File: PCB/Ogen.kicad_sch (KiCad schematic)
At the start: 17 parts, among them J1 Input, U1 PMW3360DM-T2QU, U2 TLV70019, U3 TXS0102DCU, U4 TXS0102DCU, U5 TXS0102DCU

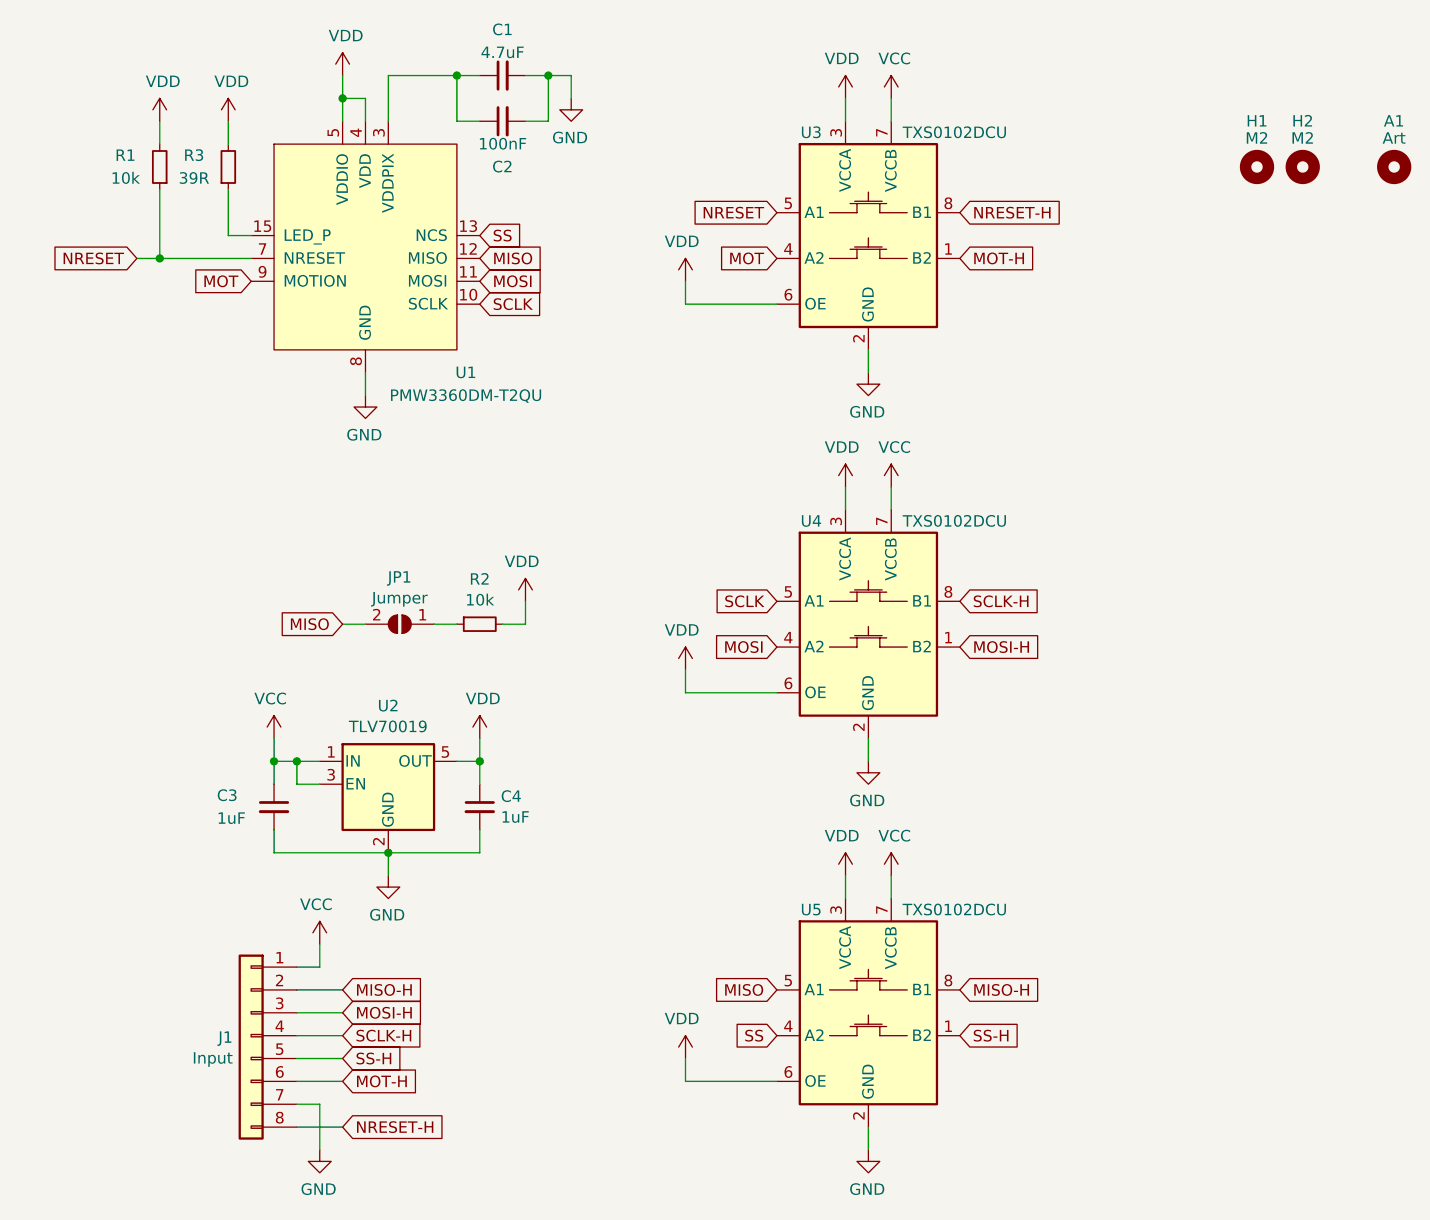
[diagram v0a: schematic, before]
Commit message: V1.0 Lite initial commit.
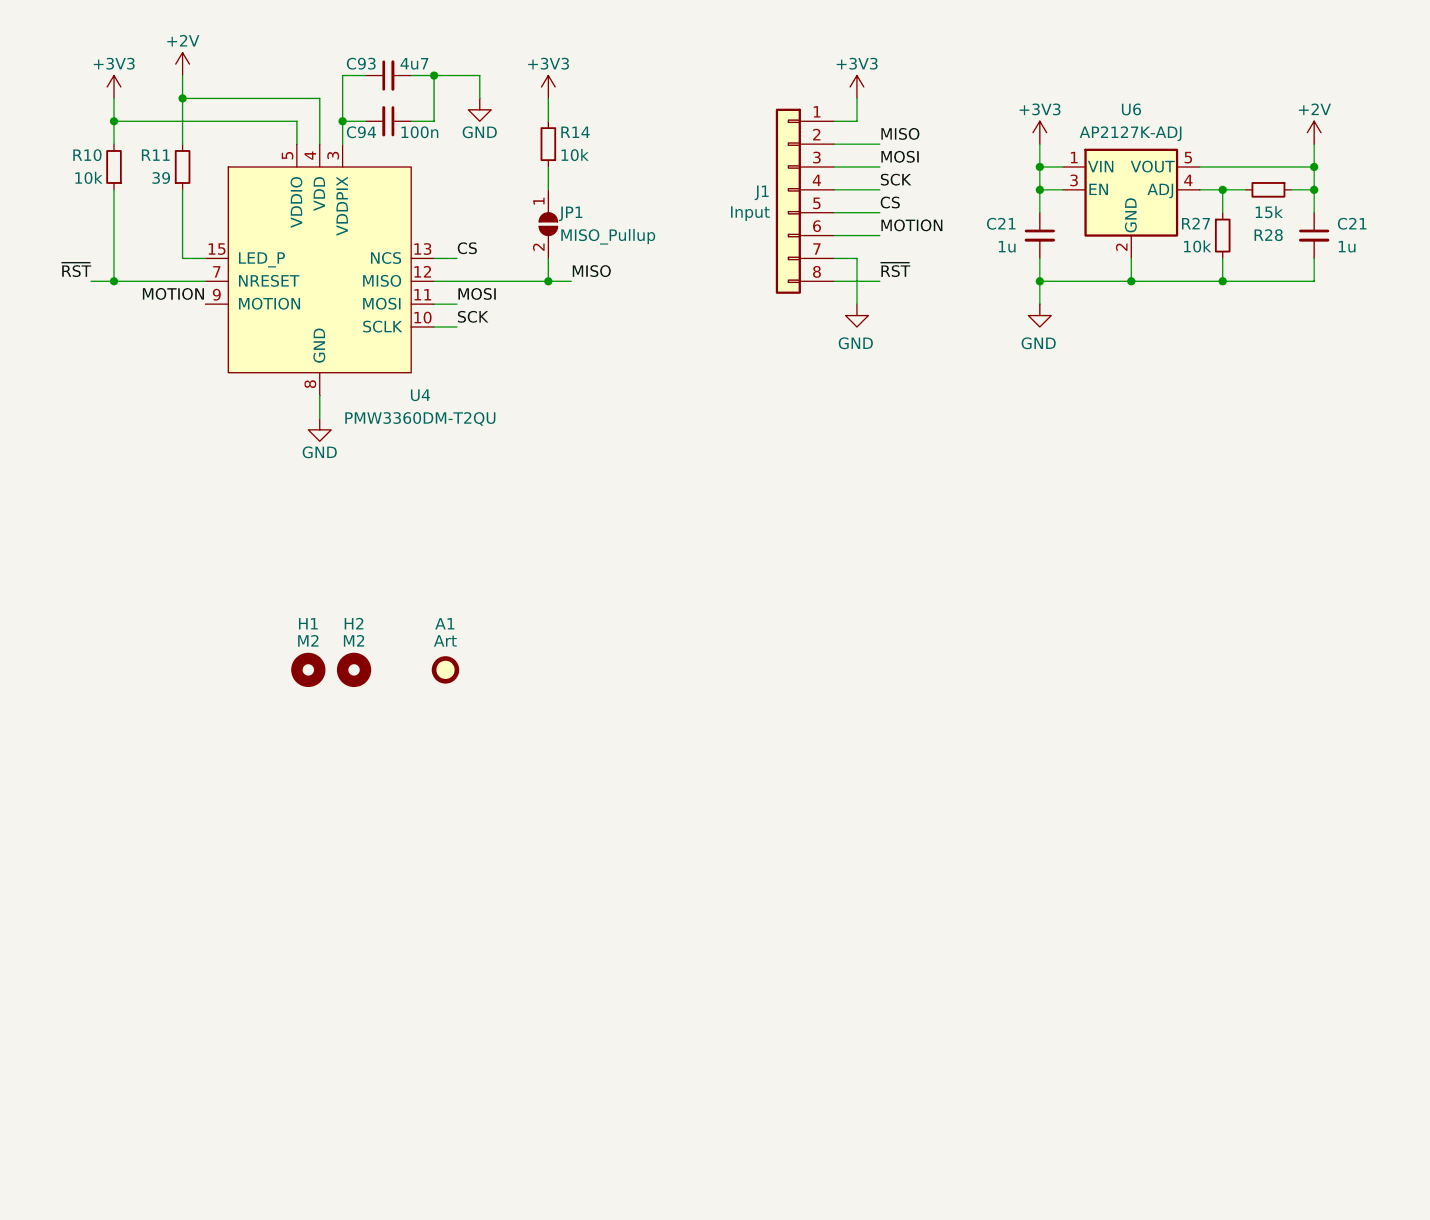
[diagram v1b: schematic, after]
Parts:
- removed C1: 4.7uF, Capacitor_SMD:C_0603_1608Metric, symbol Device:C_Small
- removed C2: 100nF, Capacitor_SMD:C_0603_1608Metric, symbol Device:C_Small
- removed C3, C4: 1uF, Capacitor_SMD:C_0603_1608Metric, symbol Device:C_Small
- removed R1, R2: 10k, Resistor_SMD:R_0603_1608Metric, symbol Device:R_Small
- removed R3: 39R, Resistor_SMD:R_0603_1608Metric, symbol Device:R_Small
- removed U1: PMW3360DM-T2QU, Ogen:IC_PMW3360DM-T2QU, symbol Ogen:PMW3360DM-T2QU
- removed U2: TLV70019, Package_TO_SOT_SMD:SOT-23-5, symbol Regulator_Linear:TLV70019_SOT23-5
- removed U3, U4, U5: TXS0102DCU, Package_SO:VSSOP-8_2.3x2mm_P0.5mm, symbol Logic_LevelTranslator:TXS0102DCU
- added C21 (x2): 1u, Capacitor_SMD:C_0402_1005Metric, symbol Device:C_Small
- added C93: 4u7, Capacitor_SMD:C_0603_1608Metric, symbol Device:C_Small
- added C94: 100n, Capacitor_SMD:C_0402_1005Metric, symbol Device:C_Small
- added R10, R14, R27: 10k, Resistor_SMD:R_0402_1005Metric, symbol Device:R_Small
- added R11: 39, Resistor_SMD:R_0402_1005Metric, symbol Device:R_Small
- added R28: 15k, Resistor_SMD:R_0402_1005Metric, symbol Device:R_Small
- added U4: PMW3360DM-T2QU, Ogen:IC_PMW3360DM-T2QU, symbol Ogen:PMW3360DM-T2QU
- added U6: AP2127K-ADJ, Package_TO_SOT_SMD:SOT-23-5, symbol Regulator_Linear:AP2127K-ADJ
- A1: footprint Ogen:Ariamelon_Logo -> Ogen:Ariamelon_Logo-CU; symbol Mechanical:MountingHole -> Mechanical:Fiducial
- J1: footprint Connector_PinHeader_2.54mm:PinHeader_1x08_P2.54mm_Vertical -> Ogen:PinHeader_1x08_P2.54mm_Vertical
- JP1: value Jumper -> MISO_Pullup; now left out of the parts list
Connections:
- net MISO-H is gone; now on net MISO: J1.2 (Pin_2)
- net MOSI-H is gone; now on net MOSI: J1.3 (Pin_3)
- net GND: now also C21.2, C21.2, C93.2, C94.1, R27.2, U4.8 (GND), U6.2 (GND)
- net MISO: now also U4.12 (MISO)
- net MOSI: now also U4.11 (MOSI)
- net at JP1.1 (A): now also R14.1
- net MOT-H renamed MOTION
- net MOTION: now also U4.9 (MOTION)
- net NRESET-H renamed ~{RST}
- net ~{RST}: now also R10.1, U4.7 (NRESET)
- net SCLK-H renamed SCK
- net SCK: now also U4.10 (SCLK)
- net SS-H renamed CS
- net CS: now also U4.13 (NCS)
- net VCC renamed +3V3
- net +3V3: now also C21.1, R10.2, R14.2, U4.5 (VDDIO), U6.1 (VIN), U6.3 (EN)
- new net: C93.1, C94.2, U4.3 (VDDPIX)
- new net: R27.1, R28.2, U6.4 (ADJ)
- new net: R11.1, U4.15 (LED_P)
- new net: U4.1 (NC), U4.14 (NC), U4.16 (NC), U4.2 (NC), U4.6 (NC)
- new net +2V: C21.1, R11.2, R28.1, U4.4 (VDD), U6.5 (VOUT)
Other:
- moved on the sheet: H1, H2
